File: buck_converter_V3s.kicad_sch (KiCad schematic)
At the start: 27 parts, among them U3001 XC6206P302MR, U3002 EA3036

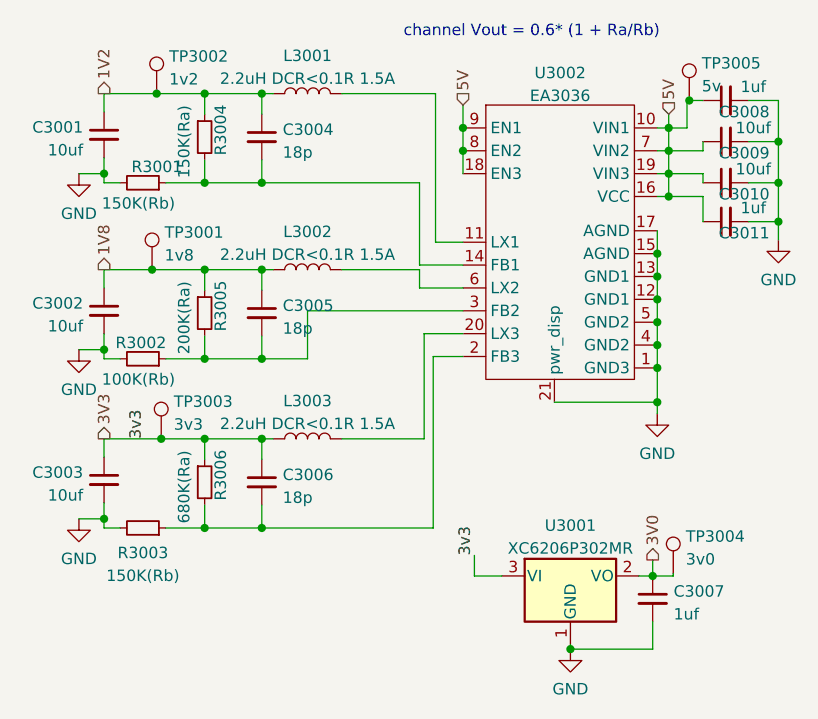
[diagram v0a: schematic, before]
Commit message: almost done
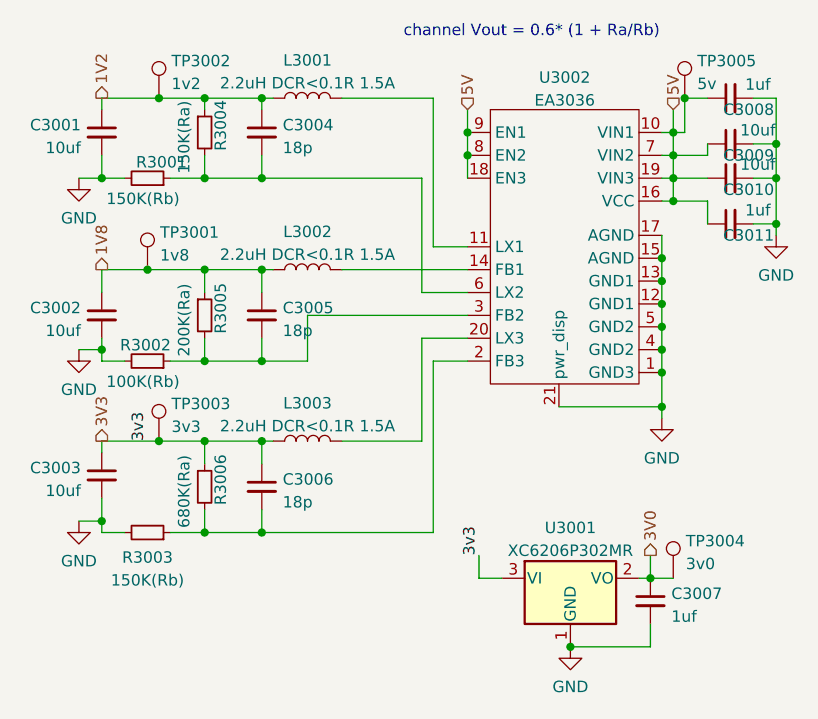
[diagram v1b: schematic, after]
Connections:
- net at C3004.2, R3001.1, R3004.2: now also U3002.6 (LX2); no longer U3002.14 (FB1)
- net at L3002.2: now also U3002.14 (FB1); no longer U3002.6 (LX2)
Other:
- moved on the sheet: C3002, C3003, C3004, C3006, C3008, C3009, C3010, C3011, L3001, R3001, R3002, R3003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
